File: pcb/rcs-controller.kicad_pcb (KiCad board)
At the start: 2 copper layers, 1 part

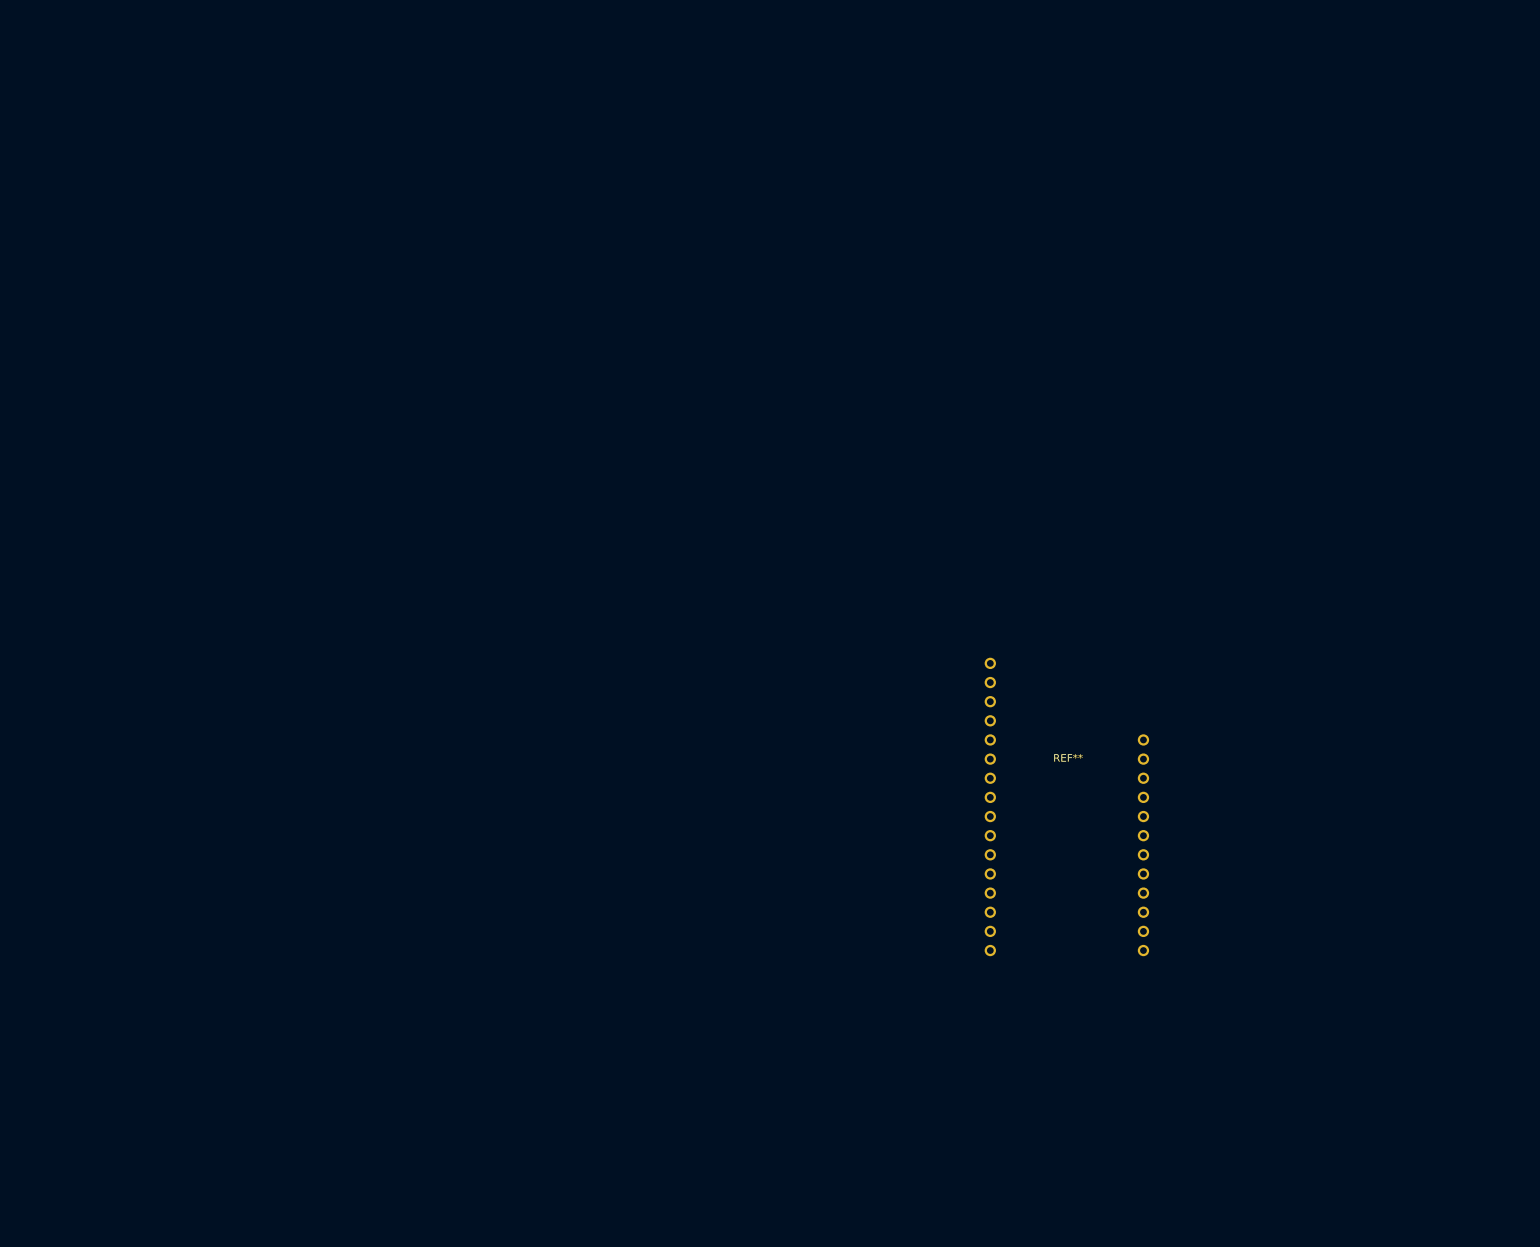
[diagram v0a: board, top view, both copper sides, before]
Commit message: First circuit board
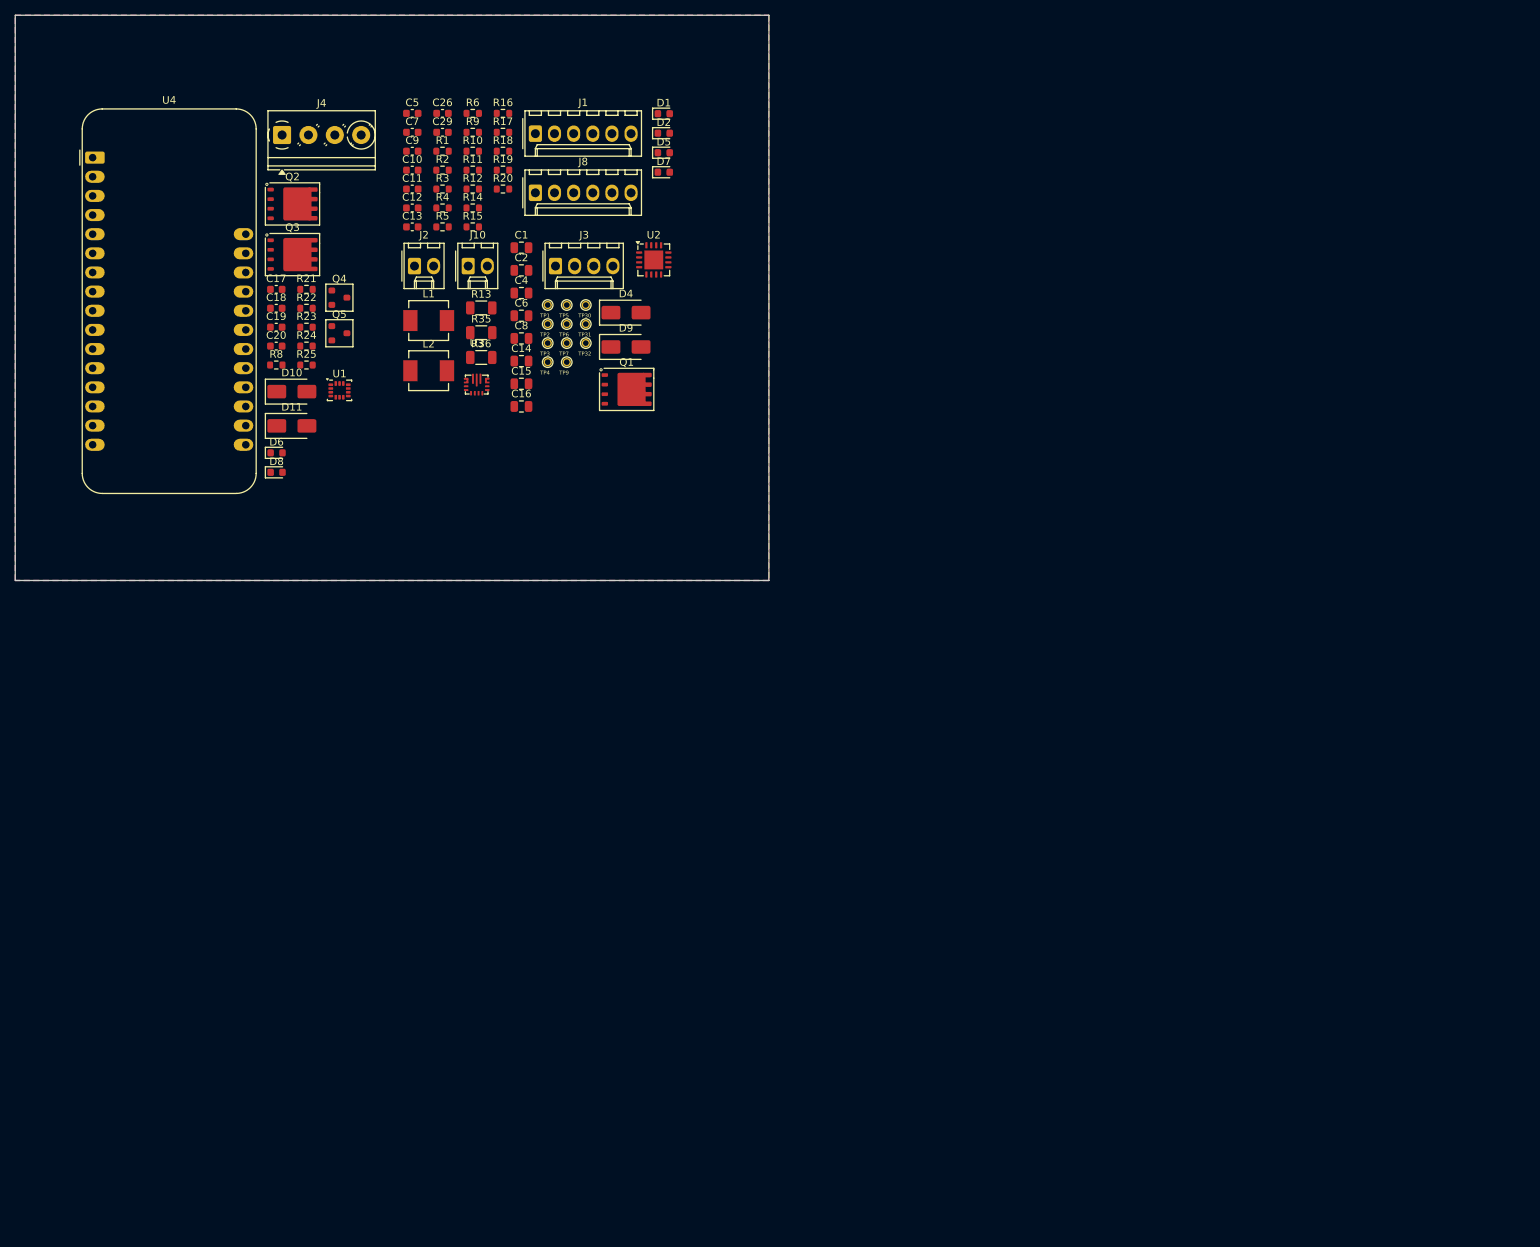
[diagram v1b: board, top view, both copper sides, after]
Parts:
- removed REF**: FeatherS3, Additional_parts:FeatherS3
- added C1: 10u, Capacitor_SMD:C_0805_2012Metric, F.Cu at (67.2, 20.8)
- added C10: 100n, Capacitor_SMD:C_0603_1608Metric, F.Cu at (52.7, 10.6)
- added C11: 2.2n, Capacitor_SMD:C_0603_1608Metric, F.Cu at (52.7, 13.1)
- added C12: 10u, Capacitor_SMD:C_0603_1608Metric, F.Cu at (52.7, 15.6)
- added C13: 2.2n, Capacitor_SMD:C_0603_1608Metric, F.Cu at (52.7, 18.1)
- added C14: 22u, Capacitor_SMD:C_0805_2012Metric, F.Cu at (67.2, 35.9)
- added C15: 22u, Capacitor_SMD:C_0805_2012Metric, F.Cu at (67.2, 38.9)
- added C16: 22u, Capacitor_SMD:C_0805_2012Metric, F.Cu at (67.2, 41.9)
- added C17: 100n, Capacitor_SMD:C_0603_1608Metric, F.Cu at (34.6, 26.4)
- added C18: 100n, Capacitor_SMD:C_0603_1608Metric, F.Cu at (34.6, 28.9)
- added C19: 100n, Capacitor_SMD:C_0603_1608Metric, F.Cu at (34.6, 31.4)
- added C2: 10u, Capacitor_SMD:C_0805_2012Metric, F.Cu at (67.2, 23.9)
- added C20: 100n, Capacitor_SMD:C_0603_1608Metric, F.Cu at (34.6, 33.9)
- added C26: 1n, Capacitor_SMD:C_0603_1608Metric, F.Cu at (56.7, 3.02)
- added C29: 100n, Capacitor_SMD:C_0603_1608Metric, F.Cu at (56.7, 5.53)
- added C4: 10u, Capacitor_SMD:C_0805_2012Metric, F.Cu at (67.2, 26.9)
- added C5: 10u, Capacitor_SMD:C_0603_1608Metric, F.Cu at (52.7, 3.02)
- added C6: 10u, Capacitor_SMD:C_0805_2012Metric, F.Cu at (67.2, 29.9)
- added C7: 100n, Capacitor_SMD:C_0603_1608Metric, F.Cu at (52.7, 5.53)
- added C8: 10u, Capacitor_SMD:C_0805_2012Metric, F.Cu at (67.2, 32.9)
- added C9: 100n, Capacitor_SMD:C_0603_1608Metric, F.Cu at (52.7, 8.04)
- added D1: GRN, LED_SMD:LED_0603_1608Metric, F.Cu at (86.1, 3.06)
- added D10: RBR5L30BDDTE25, Diode_SMD:D_SMA, F.Cu at (36.7, 39.9)
- added D11: RBR5L30BDDTE25, Diode_SMD:D_SMA, F.Cu at (36.7, 44.5)
- added D2: GRN, LED_SMD:LED_0603_1608Metric, F.Cu at (86.1, 5.65)
- added D4: RBR5L30BDDTE25, Diode_SMD:D_SMA, F.Cu at (81.0, 29.5)
- added D5: GRN, LED_SMD:LED_0603_1608Metric, F.Cu at (86.1, 8.24)
- added D6: LED, LED_SMD:LED_0603_1608Metric, F.Cu at (34.7, 48.1)
- added D7: GRN, LED_SMD:LED_0603_1608Metric, F.Cu at (86.1, 10.8)
- added D8: LED, LED_SMD:LED_0603_1608Metric, F.Cu at (34.7, 50.6)
- added D9: RBR5L30BDDTE25, Diode_SMD:D_SMA, F.Cu at (81.0, 34.0)
- added J1: 00222-32051, Connector_Molex:Molex_KK-254_AE-6410-06A_1x06_P2.54mm_Vertical, F.Cu at (69.0, 5.71)
- added J10: 0022-232021, Connector_Molex:Molex_KK-254_AE-6410-02A_1x02_P2.54mm_Vertical, F.Cu at (60.1, 23.3)
- added J2: 0022-232021, Connector_Molex:Molex_KK-254_AE-6410-02A_1x02_P2.54mm_Vertical, F.Cu at (53.0, 23.3)
- added J3: 0022-232041, Connector_Molex:Molex_KK-254_AE-6410-04A_1x04_P2.54mm_Vertical, F.Cu at (71.7, 23.3)
- added J4: Screw_Terminal_4_P3.50mm, TerminalBlock_Phoenix:TerminalBlock_Phoenix_PT-1,5-4-3.5-H_1x04_P3.50mm_Horizontal, F.Cu at (35.4, 5.89)
- added J8: 00222-32051, Connector_Molex:Molex_KK-254_AE-6410-06A_1x06_P2.54mm_Vertical, F.Cu at (69.0, 13.6)
- added L1: 1.5uH, Inductor_SMD:L_Vishay_IHLP-2020, F.Cu at (54.9, 30.5)
- added L2: 4.7uH, Inductor_SMD:L_Vishay_IHLP-2020, F.Cu at (54.9, 37.2)
- added Q1: SI7465DP-T1-E3, PCM_Package_SON_AKL:Infineon_PG-TDSON-8, F.Cu at (81.1, 39.6)
- added Q2: SI7465DP-T1-E3, PCM_Package_SON_AKL:Infineon_PG-TDSON-8, F.Cu at (36.8, 15.0)
- added Q3: SI7465DP-T1-E3, PCM_Package_SON_AKL:Infineon_PG-TDSON-8, F.Cu at (36.8, 21.8)
- added Q4: PMV45EN2, PCM_Package_TO_SOT_SMD_AKL:SOT-23, F.Cu at (43.0, 27.5)
- added Q5: PMV45EN2, PCM_Package_TO_SOT_SMD_AKL:SOT-23, F.Cu at (43.0, 32.2)
- added R1: 10k, Resistor_SMD:R_0603_1608Metric, F.Cu at (56.7, 8.04)
- added R10: 150k, Resistor_SMD:R_0603_1608Metric, F.Cu at (60.7, 8.04)
- added R11: 2.4k, Resistor_SMD:R_0603_1608Metric, F.Cu at (60.7, 10.6)
- added R12: 750, Resistor_SMD:R_0603_1608Metric, F.Cu at (60.7, 13.1)
- added R13: 100m, Resistor_SMD:R_1206_3216Metric, F.Cu at (61.8, 28.8)
- added R14: 1k, Resistor_SMD:R_0603_1608Metric, F.Cu at (60.7, 15.6)
- added R15: 1k, Resistor_SMD:R_0603_1608Metric, F.Cu at (60.7, 18.1)
- added R16: 4.7k, Resistor_SMD:R_0603_1608Metric, F.Cu at (64.7, 3.02)
- added R17: 150k, Resistor_SMD:R_0603_1608Metric, F.Cu at (64.7, 5.53)
- added R18: 10k, Resistor_SMD:R_0603_1608Metric, F.Cu at (64.7, 8.04)
- added R19: 33k, Resistor_SMD:R_0603_1608Metric, F.Cu at (64.7, 10.6)
- added R2: 4.7k, Resistor_SMD:R_0603_1608Metric, F.Cu at (56.7, 10.6)
- added R20: 10k, Resistor_SMD:R_0603_1608Metric, F.Cu at (64.7, 13.1)
- added R21: 10k, Resistor_SMD:R_0603_1608Metric, F.Cu at (38.6, 26.4)
- added R22: 10k, Resistor_SMD:R_0603_1608Metric, F.Cu at (38.6, 28.9)
- added R23: 10k, Resistor_SMD:R_0603_1608Metric, F.Cu at (38.6, 31.4)
- added R24: 1k, Resistor_SMD:R_0603_1608Metric, F.Cu at (38.6, 33.9)
- added R25: 1k, Resistor_SMD:R_0603_1608Metric, F.Cu at (38.6, 36.4)
- added R3: 4.7k, Resistor_SMD:R_0603_1608Metric, F.Cu at (56.7, 13.1)
- added R35: 60.4, Resistor_SMD:R_1206_3216Metric, F.Cu at (61.8, 32.1)
- added R36: 60.4, Resistor_SMD:R_1206_3216Metric, F.Cu at (61.8, 35.4)
- added R4: 10k, Resistor_SMD:R_0603_1608Metric, F.Cu at (56.7, 15.6)
- added R5: 10k, Resistor_SMD:R_0603_1608Metric, F.Cu at (56.7, 18.1)
- added R6: 10k, Resistor_SMD:R_0603_1608Metric, F.Cu at (60.7, 3.02)
- added R8: 10k, Resistor_SMD:R_0603_1608Metric, F.Cu at (34.6, 36.4)
- added R9: 470k, Resistor_SMD:R_0603_1608Metric, F.Cu at (60.7, 5.53)
- added TP1: Test-Point, psas-footprints:TP-through-hole-1X01, F.Cu at (70.7, 28.4)
- added TP2: Test-Point, psas-footprints:TP-through-hole-1X01, F.Cu at (70.7, 31.0)
- added TP3: Test-Point, psas-footprints:TP-through-hole-1X01, F.Cu at (70.7, 33.5)
- added TP30: Test-Point, psas-footprints:TP-through-hole-1X01, F.Cu at (75.7, 28.4)
- added TP31: Test-Point, psas-footprints:TP-through-hole-1X01, F.Cu at (75.7, 31.0)
- added TP32: Test-Point, psas-footprints:TP-through-hole-1X01, F.Cu at (75.7, 33.5)
- added TP4: Test-Point, psas-footprints:TP-through-hole-1X01, F.Cu at (70.7, 36.0)
- added TP5: Test-Point, psas-footprints:TP-through-hole-1X01, F.Cu at (73.2, 28.4)
- added TP6: Test-Point, psas-footprints:TP-through-hole-1X01, F.Cu at (73.2, 31.0)
- added TP7: Test-Point, psas-footprints:TP-through-hole-1X01, F.Cu at (73.2, 33.5)
- added TP9: Test-Point, psas-footprints:TP-through-hole-1X01, F.Cu at (73.2, 36.0)
- added U1: LSM6DSOX, Package_LGA:LGA-14_3x2.5mm_P0.5mm_LayoutBorder3x4y, F.Cu at (43.0, 39.8)
- added U2: MP26123DR-LF-Z, Package_DFN_QFN:QFN-16-1EP_4x4mm_P0.65mm_EP2.5x2.5mm, F.Cu at (84.7, 22.5)
- added U3: TPS63070, psas-footprints:U-TI-TPS63070, F.Cu at (61.2, 39.0)
- added U4: FeatherS3, Module:Adafruit_Feather, F.Cu at (10.3, 8.89)
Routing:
- added copper zone on B.Cu, net GND
- added copper zone on F.Cu, net GND
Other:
- board outline added: 100 x 75 mm

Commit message: Push to move to other machine
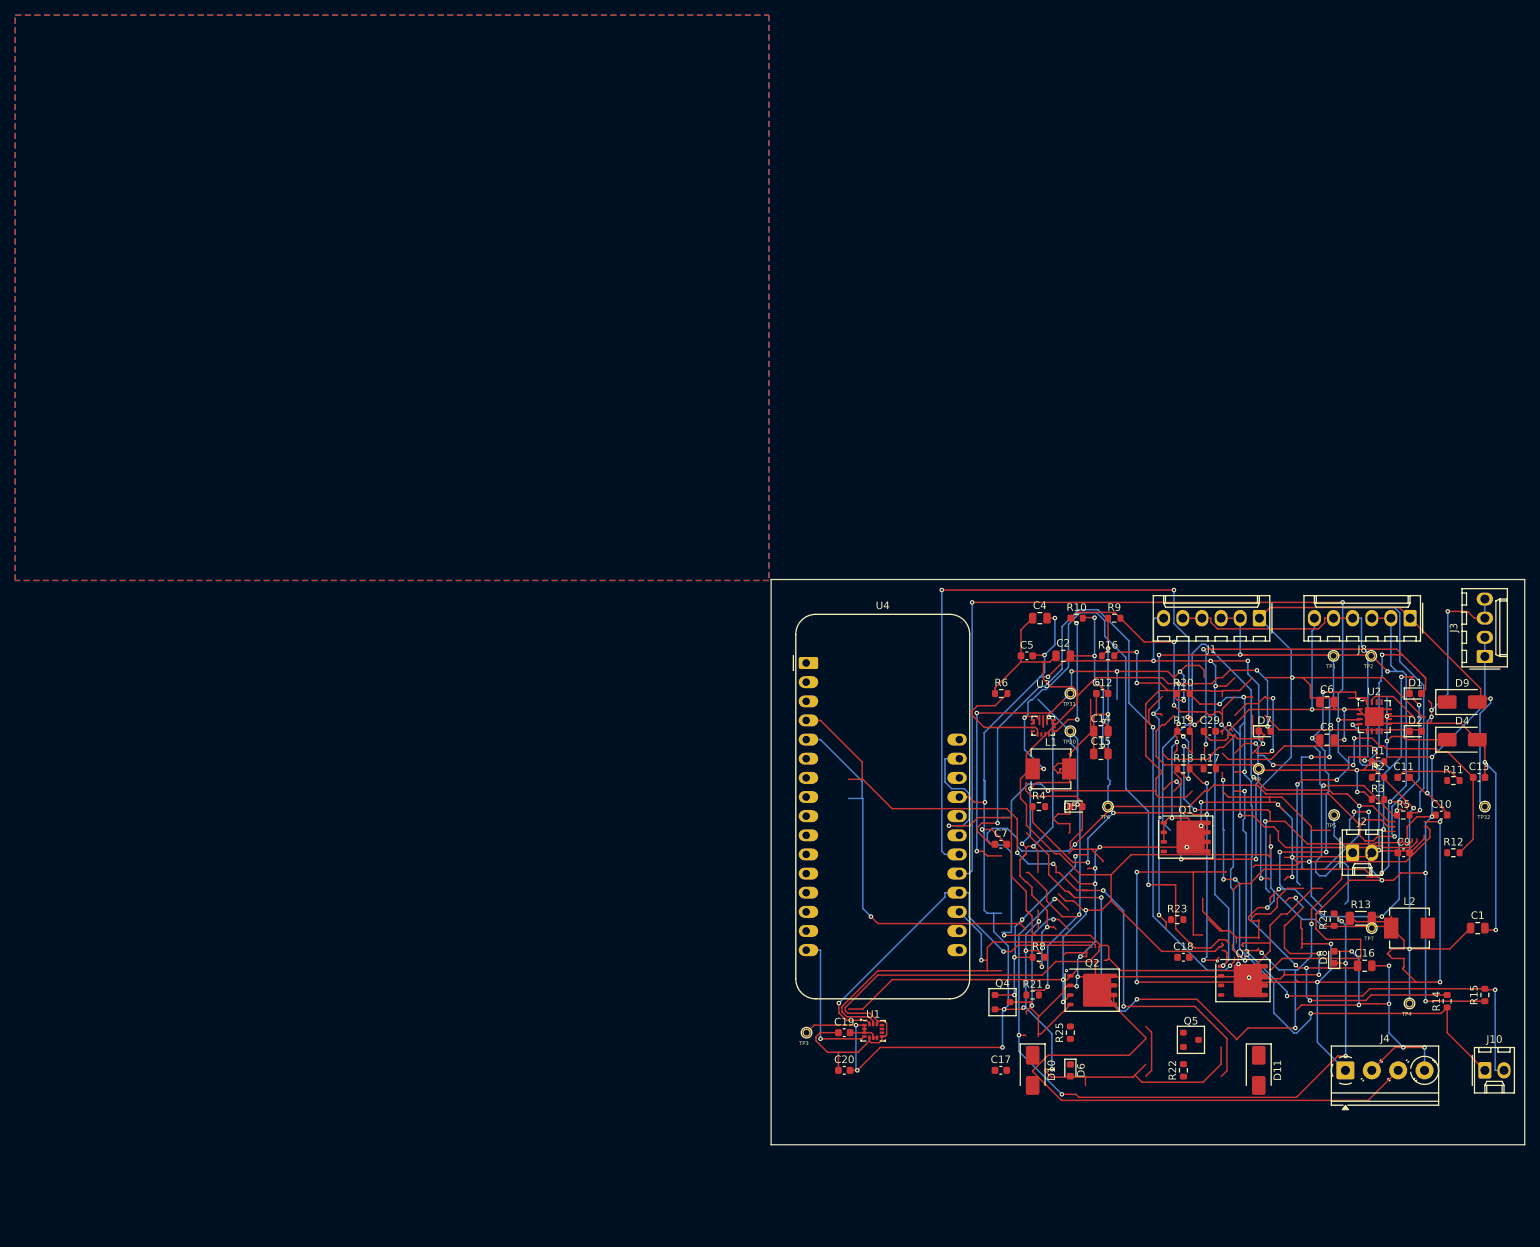
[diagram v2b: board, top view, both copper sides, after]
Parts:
- removed C26: 1n, Capacitor_SMD:C_0603_1608Metric
- removed R35, R36: 60.4, Resistor_SMD:R_1206_3216Metric
- moved J4 187.9 mm to (176.5, 130.0)
- moved J10 172.0 mm to (195.0, 130.0)
- moved R15 168.6 mm to (195.0, 120.0), turned to 90 degrees
- moved R14 166.7 mm to (190.0, 120.8), turned to 90 degrees
- moved C9 161.1 mm to (184.2, 101.1)
- moved C10 161.1 mm to (189.2, 96.1)
- moved C13 159.3 mm to (194.2, 91.1)
- moved Q3 158.7 mm to (162.9, 118.1)
- moved R12 157.1 mm to (190.8, 101.1)
- moved R24 156.2 mm to (175.0, 110.0), turned to 90 degrees
- moved C1 155.7 mm to (194.1, 111.1)
- moved D8 154.4 mm to (175.0, 115.0), turned to 90 degrees
- moved D11 154.2 mm to (165.0, 130.0), turned to -90 degrees
- moved R22 154.2 mm to (155.0, 130.0), turned to 90 degrees
- moved R11 153.3 mm to (190.8, 91.5)
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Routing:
- net GND: track 0.00 -> 530.2 mm, vias 0 -> 42
- net +3.3V: track 0.00 -> 306.5 mm, vias 0 -> 7
- net VBUS: track 0.00 -> 285.0 mm, vias 0 -> 11
- net +BATT: track 0.00 -> 243.3 mm, vias 0 -> 16
- net CANH: track 0.00 -> 177.3 mm, vias 0 -> 9
- net UMB_~{ON}: track 0.00 -> 171.5 mm, vias 0 -> 6
- net /Power/VUMB: track 0.00 -> 170.8 mm, vias 0 -> 4
- net Net-(Q2-G): track 0.00 -> 159.9 mm, vias 0 -> 13
- net Net-(D11-K): track 0.00 -> 149.1 mm, vias 0 -> 6
- net BATT_READ: track 0.00 -> 145.2 mm, vias 0 -> 6
- net Net-(Q1-G): track 0.00 -> 123.9 mm, vias 0 -> 8
- net Net-(U3-L2): track 0.00 -> 111.3 mm, vias 0 -> 8
- net Net-(U3-VAUX): track 0.00 -> 105.7 mm, vias 0 -> 3
- net Net-(D8-K): track 0.00 -> 94.8 mm, vias 0 -> 6
- net Net-(Q5-G): track 0.00 -> 93.0 mm, vias 0 -> 4
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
